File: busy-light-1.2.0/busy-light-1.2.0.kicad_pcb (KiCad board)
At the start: 4 copper layers, 40 x 92 mm, 25 parts, among them J1 Conn_01x01_Pin, J10 Conn_01x01_Pin, J11 Conn_01x01_Pin, J12 Conn_01x01_Pin, J13 Conn_01x01_Pin, J14 Conn_01x01_Pin, J15 Conn_01x01_Pin, J16 Conn_01x01_Pin, J17 Conn_01x01_Pin, J18 Conn_01x01_Pin, J2 Conn_01x01_Pin, J3 Conn_01x01_Pin, J4 Conn_01x01_Pin, J5 Conn_01x01_Pin, J6 Conn_01x01_Pin, J7 Conn_01x01_Pin, J8 Conn_01x01_Pin, J9 Conn_01x01_Pin, U1 WEMOS_D1_mini

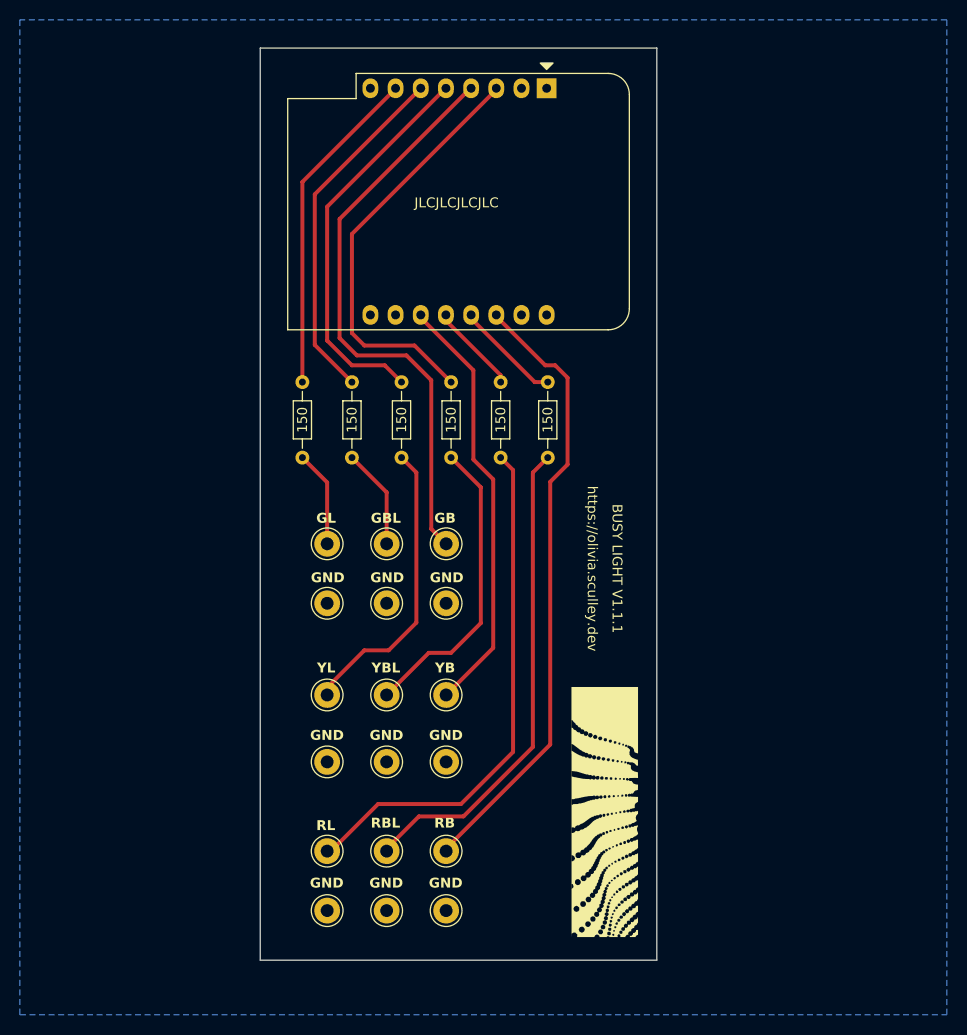
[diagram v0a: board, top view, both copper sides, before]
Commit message: update 1.2.0
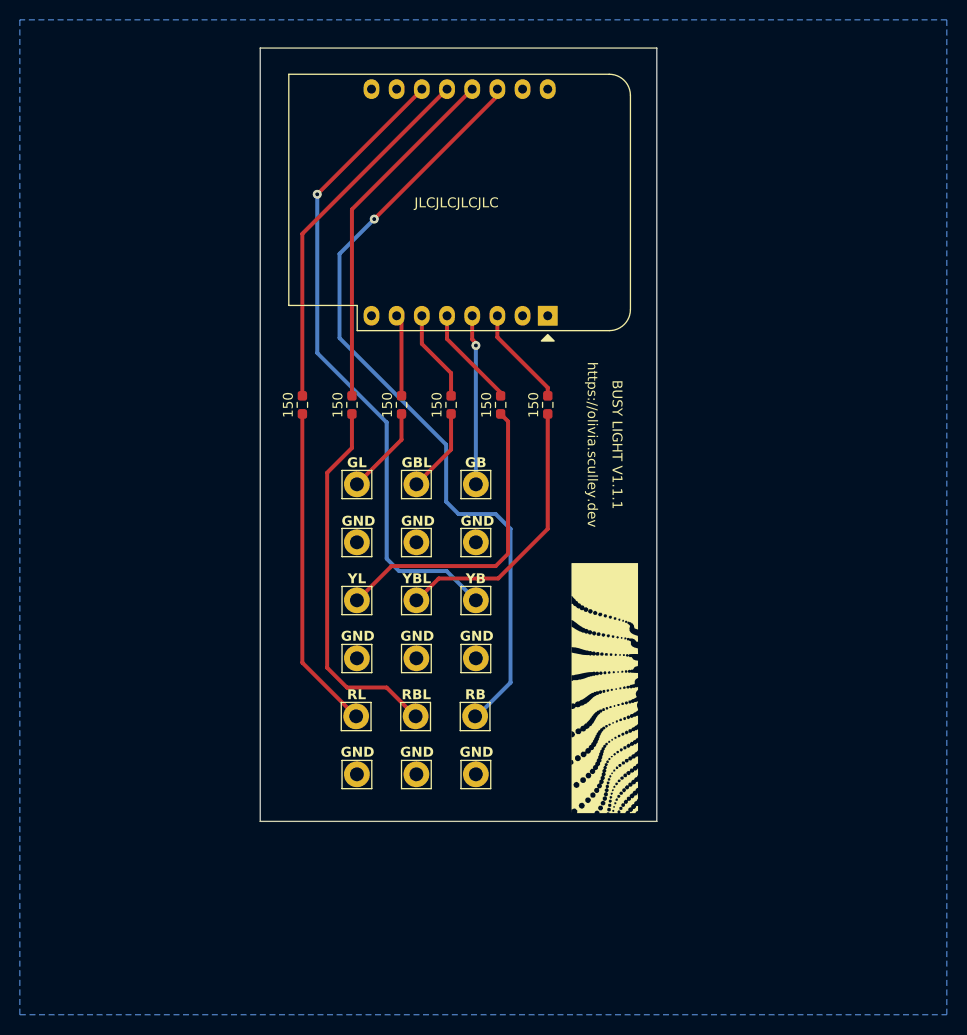
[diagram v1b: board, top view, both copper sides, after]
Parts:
- J1, J10, J11, J12, J13, J14, J15, J16, J17, J18, J2, J3, J4, J5, J6, J7, J8, J9: footprint Connector_Pin:Pin_D1.3mm_L11.0mm -> Connector_Pin:Pin_D1.4mm_L8.5mm_W2.8mm_FlatFork
- R1, R2, R3, R4, R5, R6: footprint Resistor_THT:R_Axial_DIN0204_L3.6mm_D1.6mm_P7.62mm_Horizontal -> Resistor_SMD:R_0603_1608Metric_Pad0.98x0.95mm_HandSolder
- U1: moved to B.Cu
- moved U1 22.9 mm to (133.0, 87.0), turned to 90 degrees
- moved R4 20.1 mm to (108.2, 96.0)
- moved R3 19.9 mm to (113.2, 96.0)
- moved J12 14.1 mm to (119.8, 133.2)
- moved J18 14.1 mm to (125.8, 133.2)
- moved J6 14.1 mm to (113.8, 133.2)
- moved J1 13.9 mm to (113.7, 127.4)
- moved J3 13.9 mm to (119.7, 127.4)
- moved J5 13.9 mm to (125.7, 127.4)
- moved J10 10.9 mm to (119.8, 121.5)
- moved J16 10.9 mm to (125.8, 121.5)
- moved J4 10.9 mm to (113.8, 121.5)
- moved R1 10.3 mm to (123.2, 96.0)
- moved R5 10.3 mm to (128.2, 96.0)
- moved R6 10.3 mm to (118.2, 96.0)
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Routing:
- net /GREEN BUTTON: track 58.9 -> 17.2 mm, vias 0 -> 1
- net /YELLOW BUTTON LIGHT: track 42.8 -> 10.2 mm
- net /YELLOW LIGHT: track 39.7 -> 10.3 mm
- net /RED LIGHT: track 9.06 -> 37.0 mm
- net /GREEN BUTTON LIGHT: track 35.6 -> 9.30 mm
- net /RED BUTTON LIGHT: track 10.7 -> 36.0 mm
- net /GREEN LIGHT: track 33.5 -> 8.42 mm
- net /YELLOW BUTTON: track 43.3 -> 65.7 mm, vias 0 -> 1
- net /RED LIGHT CONN: track 53.1 -> 32.8 mm
- net /RED BUTTON: track 62.7 -> 80.8 mm, vias 0 -> 1
- net /RED BUTTON LIGHT CONN: track 49.1 -> 37.7 mm
- net /YELLOW BUTTON LIGHT CONN: track 30.4 -> 28.1 mm
- net /YELLOW LIGHT CONN: track 29.7 -> 31.9 mm
- net /GREEN BUTTON LIGHT CONN: track 10.2 -> 8.55 mm
- net /GREEN LIGHT CONN: track 9.78 -> 8.96 mm
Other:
- board size 40 x 92 mm -> 40 x 78 mm
